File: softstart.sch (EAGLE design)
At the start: 9 parts, among them IC1 555

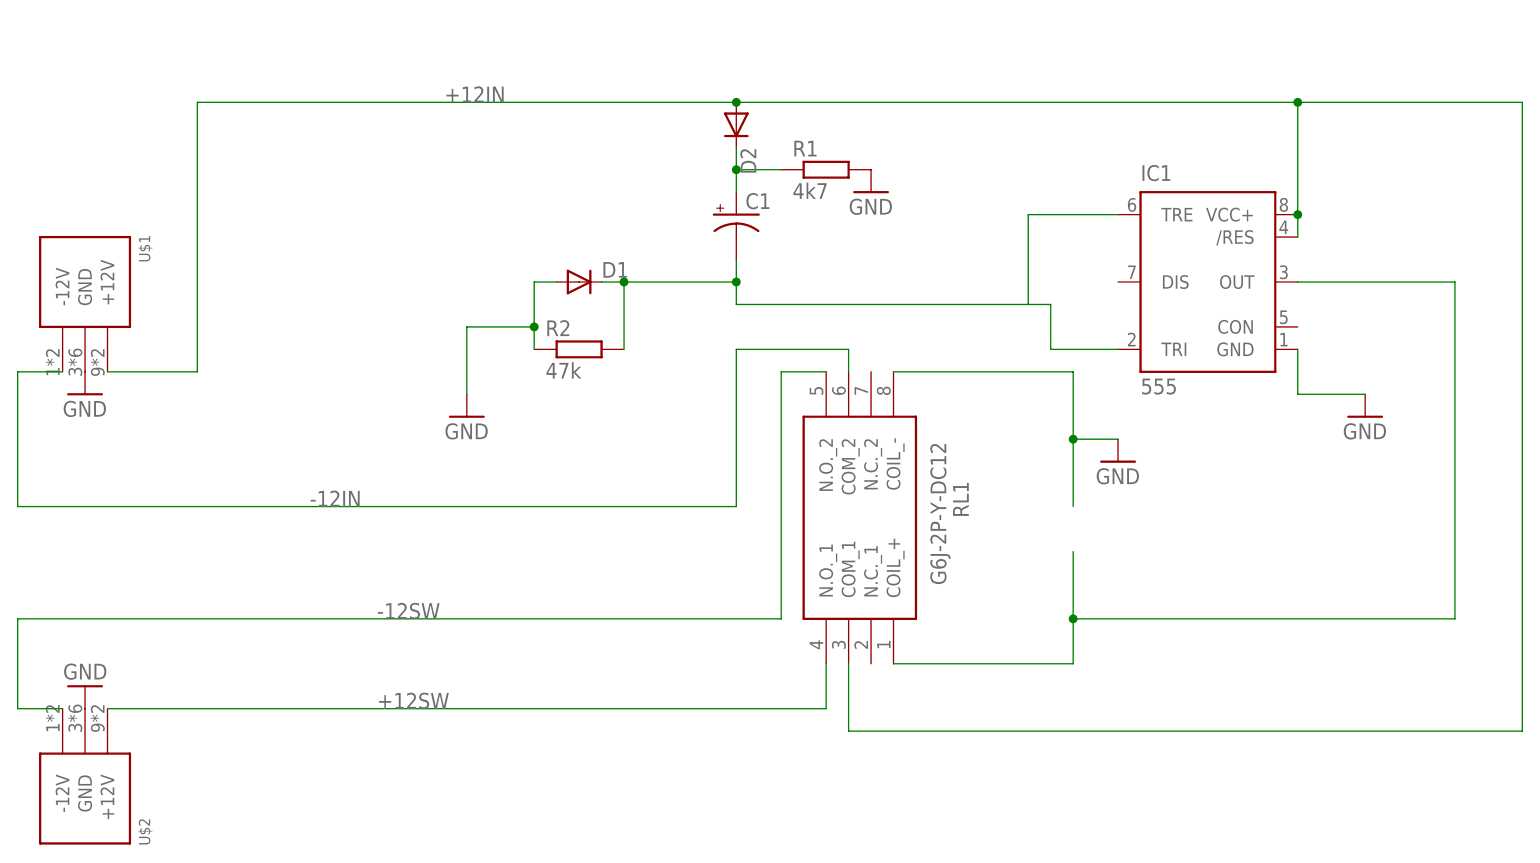
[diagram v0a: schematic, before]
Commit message: Add files via upload
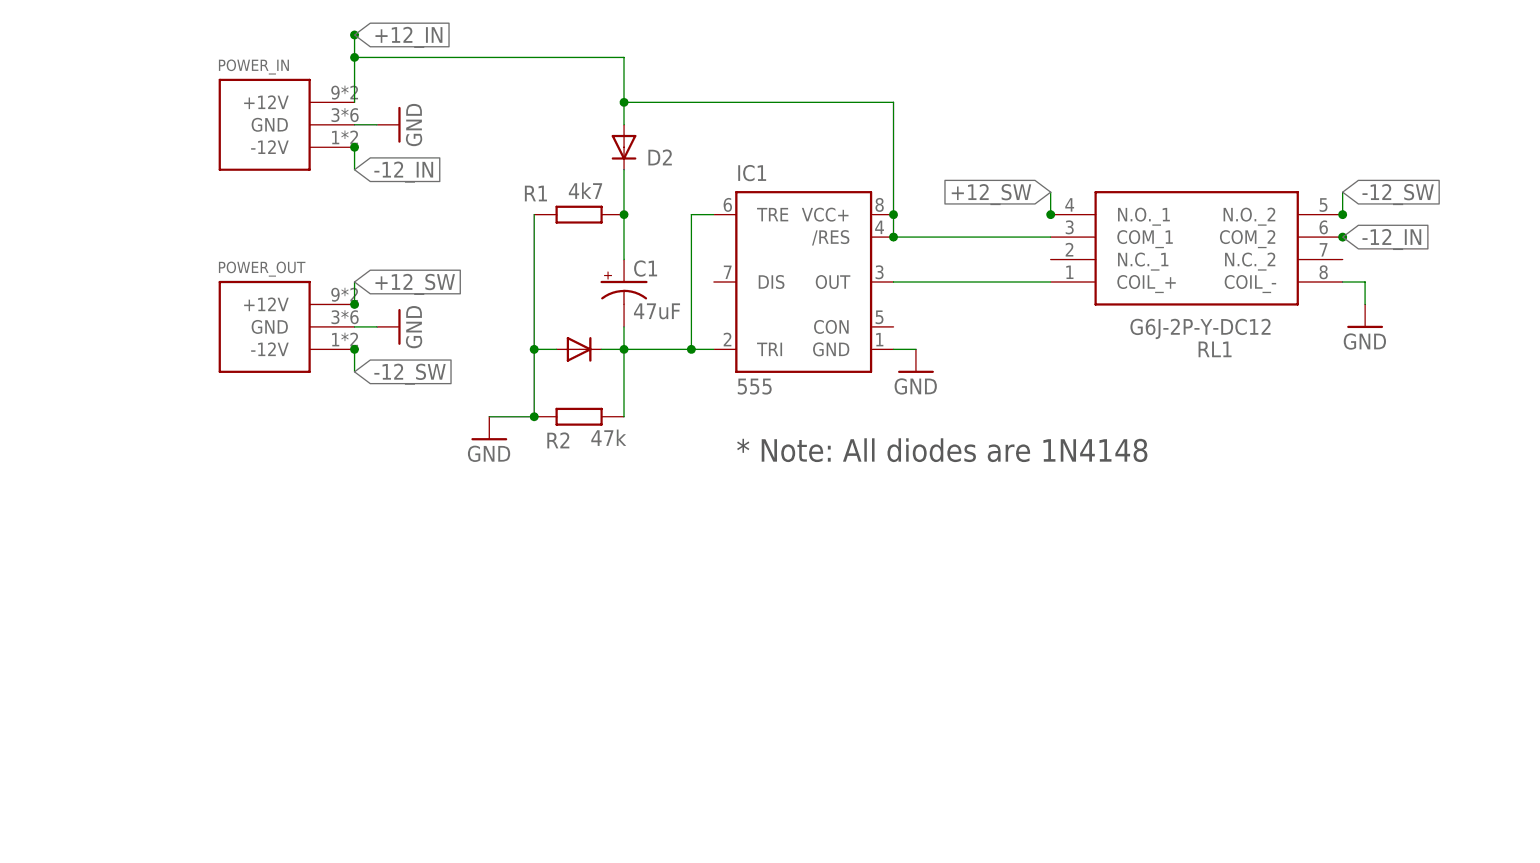
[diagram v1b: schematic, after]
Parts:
- removed U$1, U$2: RUSS_EURORACK_POWER_SIMPLE10, ES-2144 LPF Module:RUSS_EURORACK_POWER_SIMPLE10
- added POWER_IN, POWER_OUT: RUSS_EURORACK_POWER_SIMPLE10, ES-2144 LPF Module:RUSS_EURORACK_POWER_SIMPLE10
- C1: value (none) -> 47uF; device rcl:CPOL-USE5-5 -> rcl:CPOL-USTT2D6
- D1: value (none) -> 1N4001
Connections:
- removed net +12IN: D2.A, IC1./RES, IC1.VCC+, RL1.COM_1, U$1.+12V
- removed net +12SW: RL1.N.O._1, U$2.+12V
- removed net -12IN: RL1.COM_2, U$1.-12V
- removed net -12SW: RL1.N.O._2, U$2.-12V
- removed net N$2 (its old number): C1.+, D2.C, R1.1
- new net +12_IN: D2.A, IC1./RES, IC1.VCC+, POWER_IN.+12V, RL1.COM_1
- new net +12_SW: POWER_OUT.+12V, RL1.N.O._1
- new net -12_IN: POWER_IN.-12V, RL1.COM_2
- new net -12_SW: POWER_OUT.-12V, RL1.N.O._2
- new net N$1: C1.+, D2.C, R1.2
- net GND: now also POWER_IN.GND, POWER_OUT.GND, R1.1; no longer R1.2, U$1.GND, U$2.GND
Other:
- note added: "* Note: All diodes are 1N4148"
- moved on the sheet: C1, D2, IC1, R1, R2, RL1
